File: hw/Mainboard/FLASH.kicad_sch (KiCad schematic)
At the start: 5 parts, among them J26 FLASH, U22 W25Q128JVS

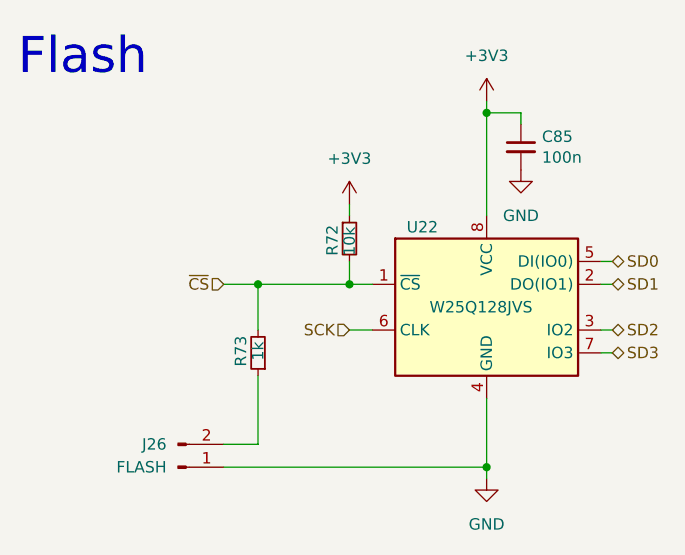
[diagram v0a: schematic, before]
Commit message: hw: 25x2 header (wip)
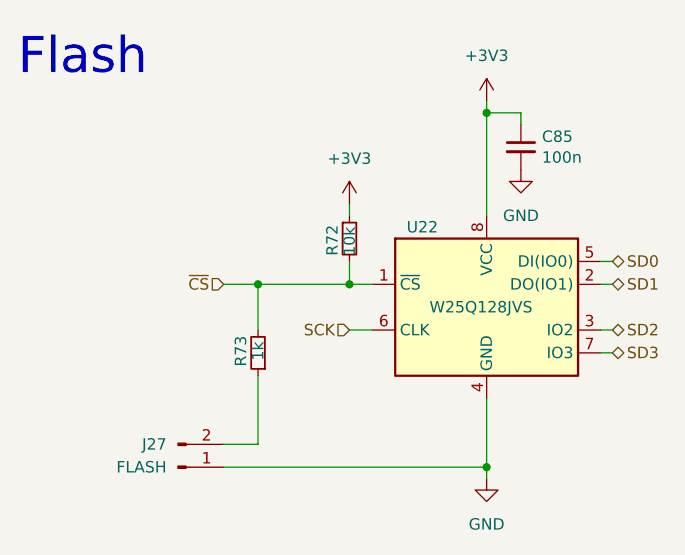
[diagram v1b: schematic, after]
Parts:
- renumbered J26 to J27
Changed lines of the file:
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@@
   (symbol (lib_id "power:GND") (at 142.24 115.57 0) (unit 1)
     (in_bom yes) (on_board yes) (fields_autoplaced)
-    (property "Reference" "#PWR0156" (id 0) (at 142.24 121.92 0)
+    (property "Reference" "#PWR0158" (id 0) (at 142.24 121.92 0)
       (effects (font (size 1.27 1.27)) hide)
     )
@@
   (symbol (lib_id "power:+3V3") (at 127 85.09 0) (unit 1)
     (in_bom yes) (on_board yes) (fields_autoplaced)
-    (property "Reference" "#PWR0155" (id 0) (at 127 88.9 0)
+    (property "Reference" "#PWR0157" (id 0) (at 127 88.9 0)
       (effects (font (size 1.27 1.27)) hide)
     )
@@
   (symbol (lib_id "Connector:Conn_01x02_Male") (at 107.95 114.3 0) (mirror x) (unit 1)
     (in_bom yes) (on_board yes) (fields_autoplaced)
-    (property "Reference" "J26" (id 0) (at 106.68 111.7599 0)
+    (property "Reference" "J27" (id 0) (at 106.68 111.7599 0)
       (effects (font (size 1.27 1.27)) (justify right))
     )
@@
   (symbol (lib_id "power:GND") (at 146.05 81.28 0) (unit 1)
     (in_bom yes) (on_board yes) (fields_autoplaced)
-    (property "Reference" "#PWR0154" (id 0) (at 146.05 87.63 0)
+    (property "Reference" "#PWR0156" (id 0) (at 146.05 87.63 0)
       (effects (font (size 1.27 1.27)) hide)
     )
@@
   (symbol (lib_id "power:+3V3") (at 142.24 73.66 0) (unit 1)
     (in_bom yes) (on_board yes) (fields_autoplaced)
-    (property "Reference" "#PWR0153" (id 0) (at 142.24 77.47 0)
+    (property "Reference" "#PWR0155" (id 0) (at 142.24 77.47 0)
       (effects (font (size 1.27 1.27)) hide)
     )

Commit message: hw: 2x config switch (wip)
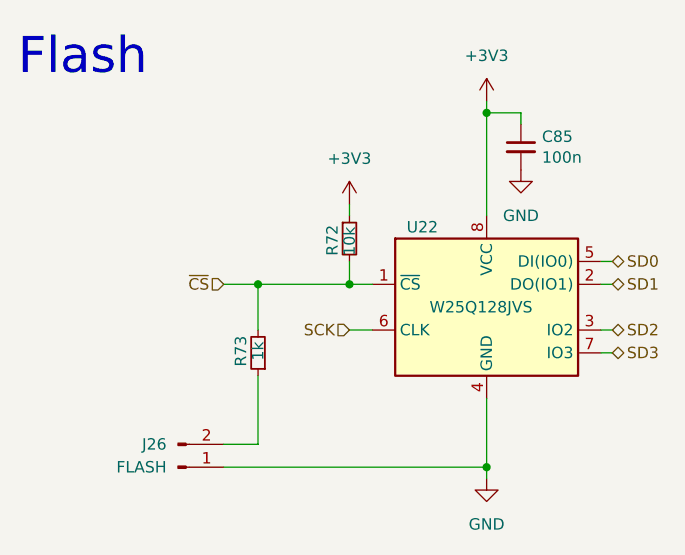
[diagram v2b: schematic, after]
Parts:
- renumbered J27 to J26
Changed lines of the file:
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@@
   (symbol (lib_id "power:GND") (at 142.24 115.57 0) (unit 1)
     (in_bom yes) (on_board yes) (fields_autoplaced)
-    (property "Reference" "#PWR0158" (id 0) (at 142.24 121.92 0)
+    (property "Reference" "#PWR0164" (id 0) (at 142.24 121.92 0)
       (effects (font (size 1.27 1.27)) hide)
     )
@@
   (symbol (lib_id "power:+3V3") (at 127 85.09 0) (unit 1)
     (in_bom yes) (on_board yes) (fields_autoplaced)
-    (property "Reference" "#PWR0157" (id 0) (at 127 88.9 0)
+    (property "Reference" "#PWR0163" (id 0) (at 127 88.9 0)
       (effects (font (size 1.27 1.27)) hide)
     )
@@
   (symbol (lib_id "Connector:Conn_01x02_Male") (at 107.95 114.3 0) (mirror x) (unit 1)
     (in_bom yes) (on_board yes) (fields_autoplaced)
-    (property "Reference" "J27" (id 0) (at 106.68 111.7599 0)
+    (property "Reference" "J26" (id 0) (at 106.68 111.7599 0)
       (effects (font (size 1.27 1.27)) (justify right))
     )
@@
   (symbol (lib_id "power:GND") (at 146.05 81.28 0) (unit 1)
     (in_bom yes) (on_board yes) (fields_autoplaced)
-    (property "Reference" "#PWR0156" (id 0) (at 146.05 87.63 0)
+    (property "Reference" "#PWR0162" (id 0) (at 146.05 87.63 0)
       (effects (font (size 1.27 1.27)) hide)
     )
@@
   (symbol (lib_id "power:+3V3") (at 142.24 73.66 0) (unit 1)
     (in_bom yes) (on_board yes) (fields_autoplaced)
-    (property "Reference" "#PWR0155" (id 0) (at 142.24 77.47 0)
+    (property "Reference" "#PWR0161" (id 0) (at 142.24 77.47 0)
       (effects (font (size 1.27 1.27)) hide)
     )
